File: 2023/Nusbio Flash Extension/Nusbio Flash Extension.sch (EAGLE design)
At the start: 8 parts

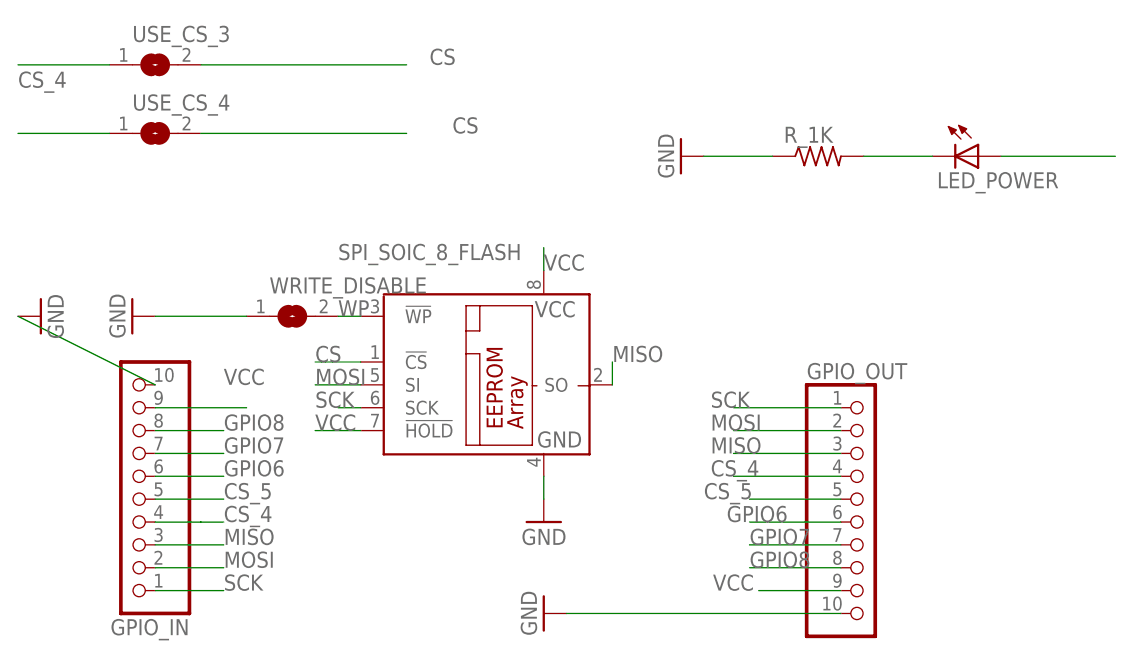
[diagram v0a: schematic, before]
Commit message: update
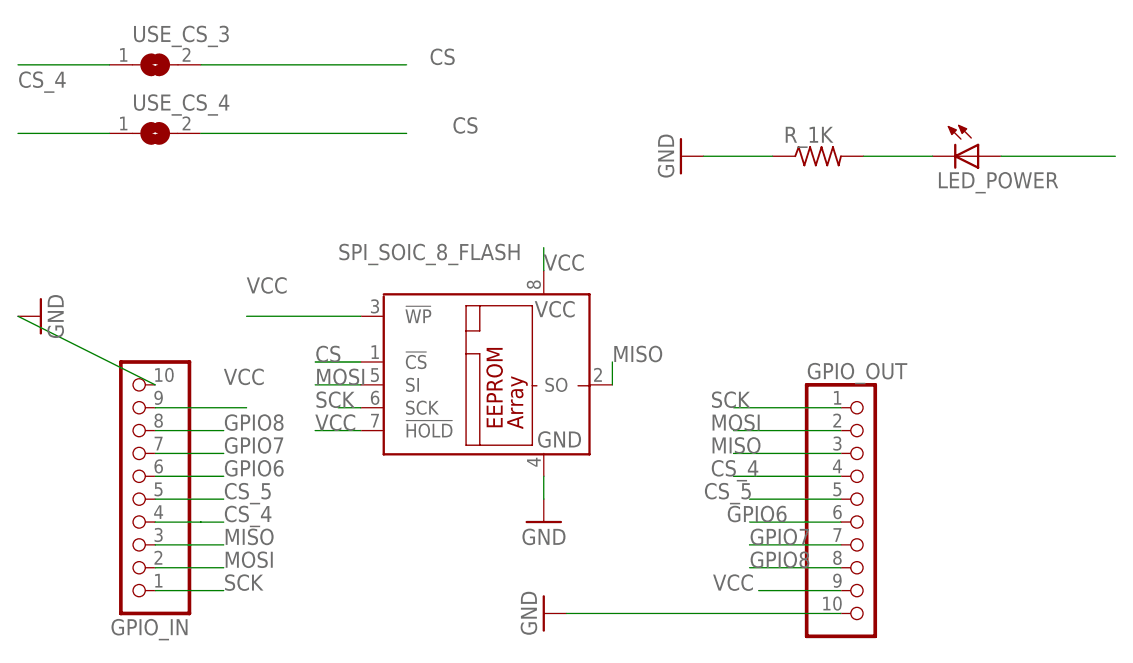
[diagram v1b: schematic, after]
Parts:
- removed WRITE_DISABLE: (no value), microbuilder:SOLDERJUMPERREFLOW
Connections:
- removed net WP: SPI_SOIC_8_FLASH.!WP, WRITE_DISABLE.2
- net GND: no longer WRITE_DISABLE.1
- net VCC: now also SPI_SOIC_8_FLASH.!WP
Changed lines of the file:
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@@
 <part name="SPI_SOIC_8_FLASH" library="microchip" deviceset="25*" device="SN" technology="AA080"/>
 <part name="GND2" library="supply1" deviceset="GND" device=""/>
-<part name="WRITE_DISABLE" library="microbuilder" deviceset="SOLDERJUMPER" device="REFLOW"/>
 <part name="R_1K" library="adafruit" deviceset="R-US_" device="R1206"/>
 <part name="LED_POWER" library="adafruit" deviceset="LED" device="SMT1206"/>
@@
 <part name="USE_CS_3" library="microbuilder" deviceset="SOLDERJUMPER" device="REFLOW"/>
 <part name="USE_CS_4" library="microbuilder" deviceset="SOLDERJUMPER" device="REFLOW"/>
-<part name="GND5" library="supply1" deviceset="GND" device=""/>
 </parts>
 <sheets>
@@
 <attribute name="VALUE" x="66.04" y="50.8" size="1.778" layer="96" rot="MR0"/>
 </instance>
-<instance part="WRITE_DISABLE" gate="1" x="35.56" y="76.2" smashed="yes">
-<attribute name="NAME" x="33.02" y="78.74" size="1.778" layer="95"/>
-<attribute name="VALUE" x="33.02" y="72.39" size="1.778" layer="96"/>
-</instance>
 <instance part="R_1K" gate="G$1" x="93.98" y="93.98" smashed="yes">
 <attribute name="NAME" x="90.17" y="95.4786" size="1.778" layer="95"/>
@@
 <attribute name="NAME" x="17.78" y="99.06" size="1.778" layer="95"/>
 <attribute name="VALUE" x="17.78" y="92.71" size="1.778" layer="96"/>
-</instance>
-<instance part="GND5" gate="1" x="17.78" y="76.2" smashed="yes" rot="R270">
-<attribute name="VALUE" x="15.24" y="78.74" size="1.778" layer="96" rot="R270"/>
 </instance>
 </instances>
@@
 <wire x1="88.9" y1="93.98" x2="81.28" y2="93.98" width="0.1524" layer="91"/>
 </segment>
-<segment>
-<pinref part="GND5" gate="1" pin="GND"/>
-<pinref part="WRITE_DISABLE" gate="1" pin="1"/>
-<wire x1="20.32" y1="76.2" x2="30.48" y2="76.2" width="0.1524" layer="91"/>
-</segment>
 </net>
 <net name="VCC" class="0">
@@
 <pinref part="LED_POWER" gate="G$1" pin="A"/>
 <wire x1="114.3" y1="93.98" x2="127" y2="93.98" width="0.1524" layer="91"/>
+</segment>
+<segment>
+<pinref part="SPI_SOIC_8_FLASH" gate="G$1" pin="!WP"/>
+<wire x1="43.18" y1="76.2" x2="30.48" y2="76.2" width="0.1524" layer="91"/>
+<label x="30.48" y="78.74" size="1.778" layer="95"/>
 </segment>
 </net>
@@
 </segment>
 </net>
-<net name="WP" class="0">
-<segment>
-<pinref part="WRITE_DISABLE" gate="1" pin="2"/>
-<pinref part="SPI_SOIC_8_FLASH" gate="G$1" pin="!WP"/>
-<wire x1="40.64" y1="76.2" x2="43.18" y2="76.2" width="0.1524" layer="91"/>
-<label x="40.64" y="76.2" size="1.778" layer="95"/>
-</segment>
-</net>
